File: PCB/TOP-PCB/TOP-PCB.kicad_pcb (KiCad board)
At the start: 2 copper layers, 35 x 35 mm, 9 parts, among them J1 Conn_01x04_Pin, J2 Conn_01x04_Pin, J3 Conn_01x12_Pin, Q1 QM6006D

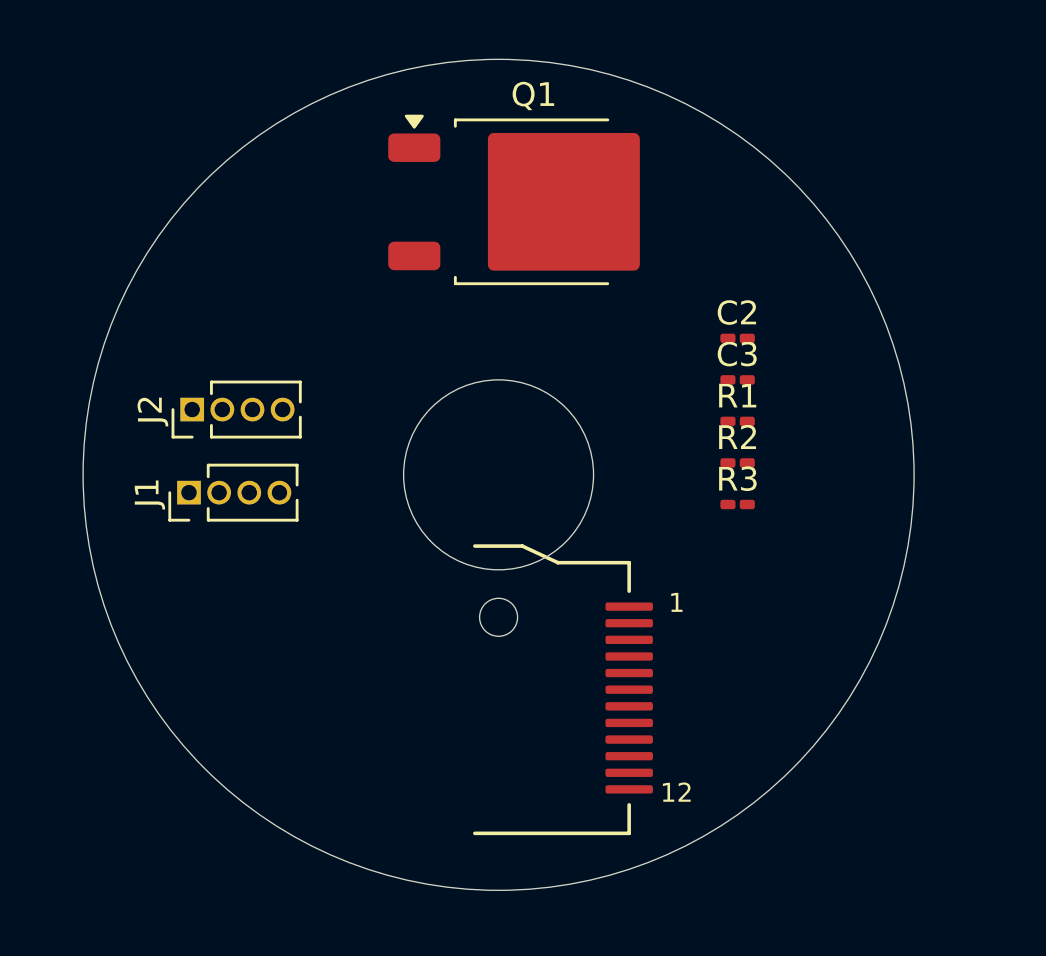
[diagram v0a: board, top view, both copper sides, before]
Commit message: TOP-PCB ready
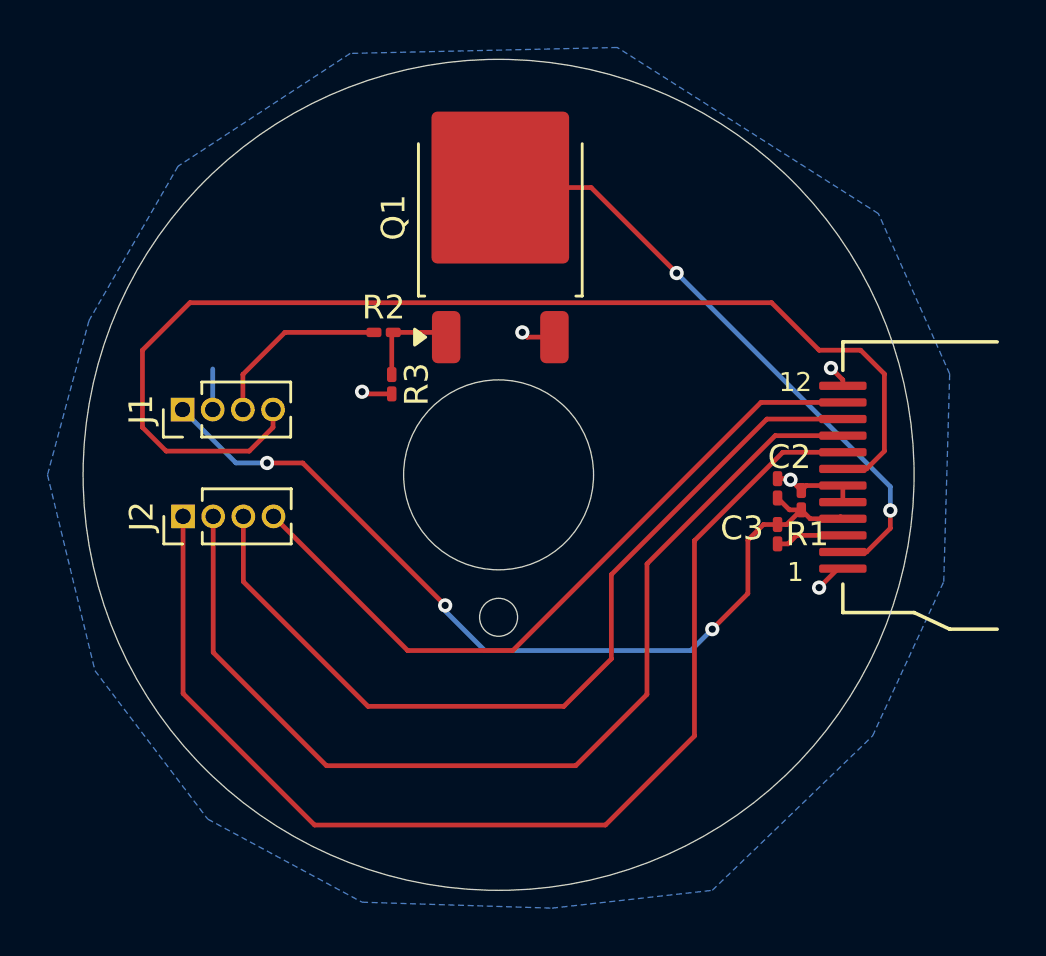
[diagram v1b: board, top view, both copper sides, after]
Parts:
- moved R2 15.9 mm to (145.7, 94.5)
- moved R3 15.4 mm to (146.0, 96.7), turned to -90 degrees
- moved J3 12.9 mm to (165.0, 100.6), turned to 180 degrees
- moved C2 6.54 mm to (162.2, 101.1), turned to 90 degrees
- moved C3 5.73 mm to (163.2, 101.6), turned to 90 degrees
- moved R1 5.04 mm to (162.2, 103.0), turned to -90 degrees
- moved J2 4.52 mm to (137.2, 102.2)
- moved J1 3.51 mm to (137.2, 97.8)
- moved Q1 1.56 mm to (150.6, 89.7), turned to 90 degrees
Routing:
- net DC: track 0.00 -> 49.0 mm
- net nCS: track 0.00 -> 48.9 mm
- net SCK: track 0.00 -> 43.2 mm
- net +3.3V: track 0.00 -> 37.4 mm, vias 0 -> 3
- net MOSI: track 0.00 -> 37.3 mm
- net nRESET: track 0.00 -> 30.6 mm
- net LEDK: track 0.00 -> 25.8 mm, vias 0 -> 2
- net GND: track 0.00 -> 10.5 mm, vias 0 -> 5
- net BACKLIGH_EN: track 0.00 -> 7.73 mm
- net Net-(Q1-G): track 0.00 -> 4.11 mm
- net LEDA: track 0.00 -> 2.92 mm
- added copper zone on B.Cu, net GND
